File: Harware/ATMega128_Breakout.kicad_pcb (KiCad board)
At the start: 2 copper layers, 40.5 x 75.1 mm, 20 parts, among them IC1 ATMEGA128-A, J1 SIL8, J2 SIL8, P1 CONN_10, P2 CONN_10, P3 CONN_10, P4 CONN_10, P6 CONN_7, P8 CONN_5X2, SW1 rst, X1 16Mhz

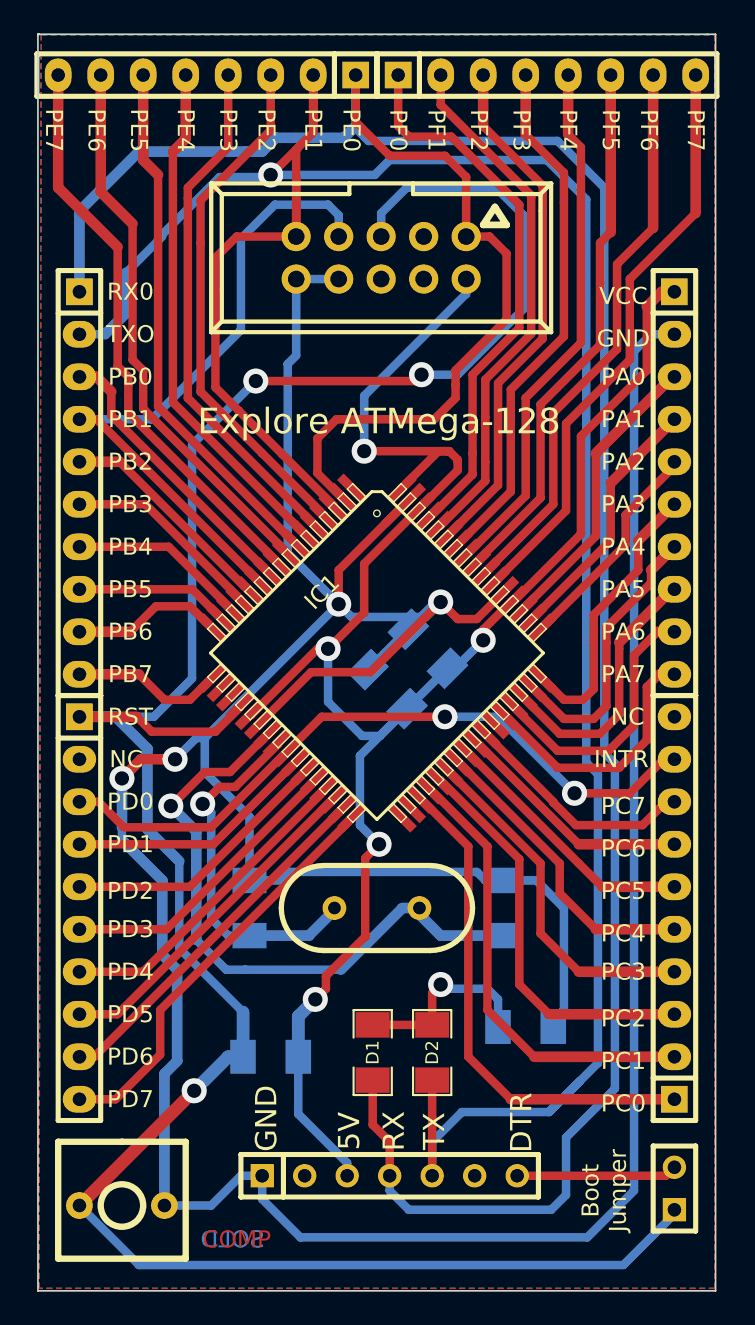
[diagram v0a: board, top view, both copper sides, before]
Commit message: added final files
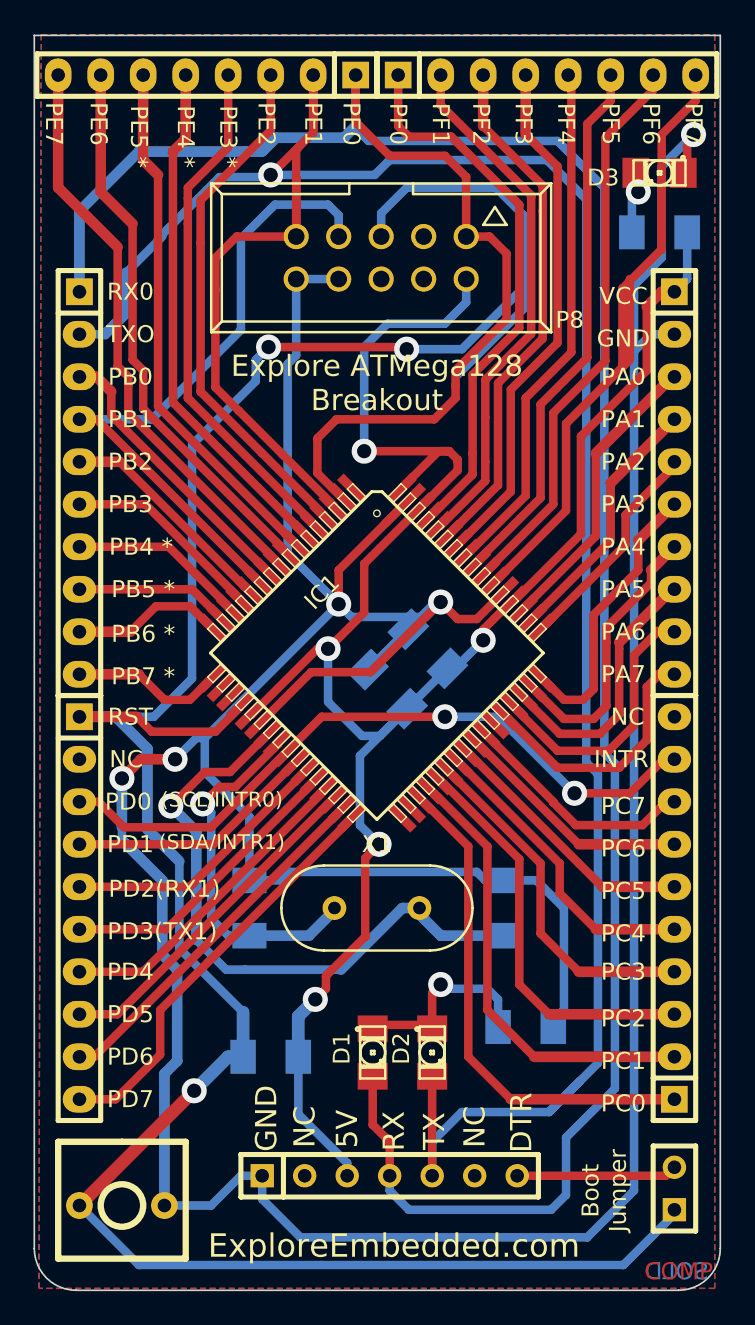
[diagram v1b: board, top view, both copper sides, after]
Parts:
- added D3: LED, ex:LED-1206_NEW, F.Cu at (94.9, 45.2)
- added LOGO: , EE:LOGO (2), B.Cu at (83.0, 56.5)
- added R3: 470r, SM1206, B.Cu at (94.9, 48.8)
- D1, D2: footprint SM1206 -> ex:LED-1206_NEW
- P8: footprint VASCH5x2 -> Connect:VASCH5x2
- X1: footprint HC-49V -> Discret:HC-49V
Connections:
- IC1 pad 1: (no net) -> Net-(IC1-Pad1)
- IC1 pad 18: (no net) -> Net-(IC1-Pad18)
- IC1 pad 19: (no net) -> Net-(IC1-Pad19)
- IC1 pad 33: (no net) -> Net-(IC1-Pad33)
- IC1 pad 34: (no net) -> Net-(IC1-Pad34)
- IC1 pad 43: (no net) -> Net-(IC1-Pad43)
- P2 pad 2: (no net) -> Net-(P2-Pad2)
- P4 pad 10: (no net) -> Net-(P4-Pad10)
- P6 pad 2: (no net) -> Net-(P6-Pad2)
- P6 pad 6: (no net) -> Net-(P6-Pad6)
- P8 pad 3: (no net) -> Net-(P8-Pad3)
- P8 pad 4: (no net) -> Net-(P8-Pad4)
- P8 pad 6: (no net) -> Net-(P8-Pad6)
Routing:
- net GND: track 232.0 -> 248.9 mm, vias 4 -> 5
- net /RST: track 149.9 -> 159.6 mm
- net /+5V: track 117.8 -> 123.7 mm
- net Net-(IC1-Pad54): track 35.3 -> 40.7 mm
- net Net-(D3-Pad1): track 0.00 -> 3.87 mm, vias 0 -> 1
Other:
- board size 40.5 x 75.1 mm -> 41 x 75 mm
- board text added: "(SCL/INTR0)"
- board text added: "(SDA/INTR1)"
- board text added: "Explore ATMega128 Breakout"
- board text added: "ExploreEmbedded.com"
- board text added: "PB4 *"
- board text added: "PB5 *"
- board text added: "PB6 *"
- board text added: "PB7 *"
- board text added: "PD2(RX1)"
- board text added: "PD3(TX1)"
- board text added: "PE3 *"
- board text added: "PE4 *"
- board text added: "PE5 *"
- board text removed: "Explore ATMega-128"
- board text removed: "PB4"
- board text removed: "PB5"
- board text removed: "PB6"
- board text removed: "PB7"
- board text removed: "PD2"
- board text removed: "PD3"
- board text removed: "PE3"
- board text removed: "PE4"
- board text removed: "PE5"
